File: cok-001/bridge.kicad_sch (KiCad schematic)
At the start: 48 parts, among them U7301 CXD9208GP

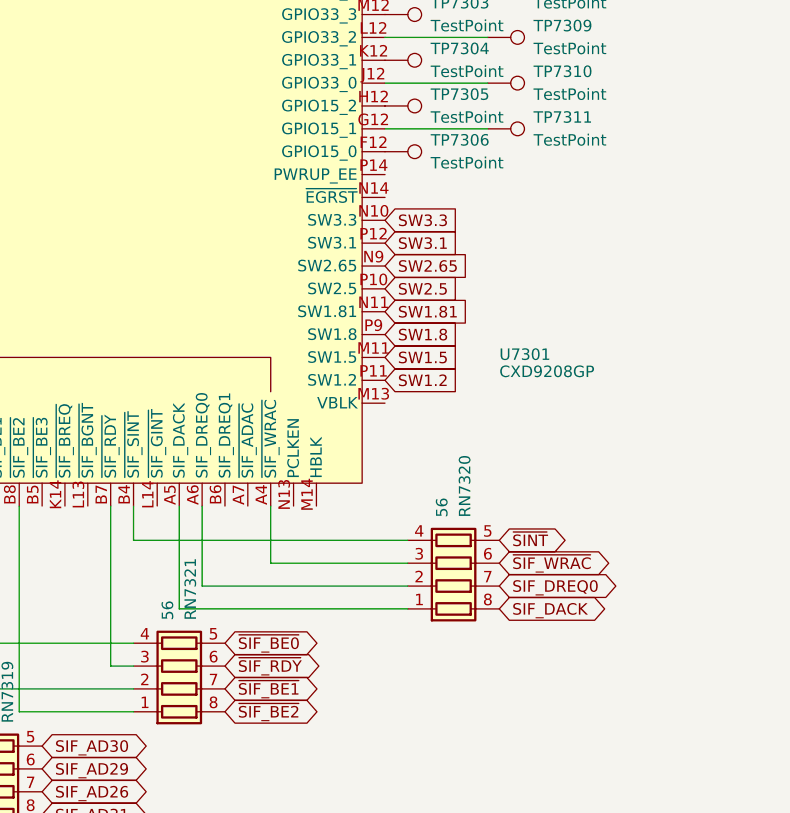
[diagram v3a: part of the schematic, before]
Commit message: ps2
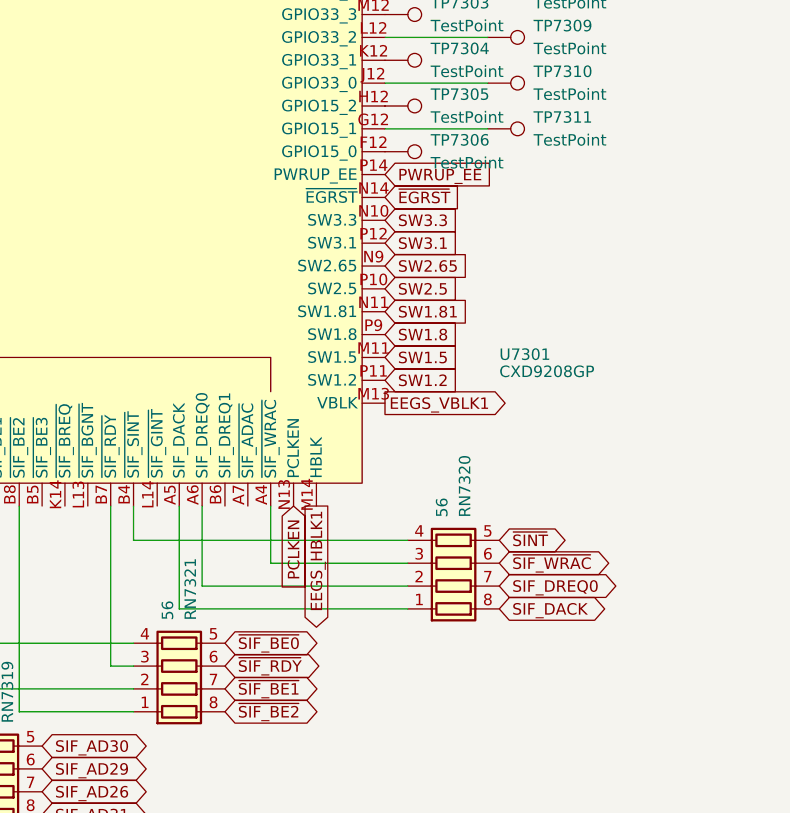
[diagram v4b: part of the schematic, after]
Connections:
- net EEGS_VBLK1: now reaches U7301.M13 (VBLK)
- net EEGS_HBLK1: now reaches U7301.M14 (HBLK)
- net PCLKEN: now reaches U7301.N13 (PCLKEN)
- net ~{EGRST}: now reaches U7301.N14 (~{EGRST})
- net PWRUP_EE: now reaches U7301.P14 (PWRUP_EE)
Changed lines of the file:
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@@
+		)
+	)
+	(global_label "EEGS_HBLK1"
+		(shape output)
+		(at 228.6 166.37 270)
+		(fields_autoplaced yes)
+		(effects
+			(font
+				(size 1.27 1.27)
+			)
+			(justify right)
+		)
+		(property "Intersheetrefs" "${INTERSHEET_REFS}"
+			(at 228.6 181.2084 90)
+			(effects
+				(font
+					(size 1.27 1.27)
+				)
+				(justify right)
+				(hide yes)
+			)
 		)
 	)
@@
 		)
 	)
+	(global_label "EEGS_VBLK1"
+		(shape output)
+		(at 236.22 154.94 0)
+		(fields_autoplaced yes)
+		(effects
+			(font
+				(size 1.27 1.27)
+			)
+			(justify left)
+		)
+		(property "Intersheetrefs" "${INTERSHEET_REFS}"
+			(at 250.8165 154.94 0)
+			(effects
+				(font
+					(size 1.27 1.27)
+				)
+				(justify left)
+				(hide yes)
+			)
+		)
+	)
 	(global_label "SIF_DACK"
 		(shape bidirectional)
@@
 		(property "Intersheetrefs" "${INTERSHEET_REFS}"
 			(at 73.66 1.3464 90)
+			(effects
+				(font
+					(size 1.27 1.27)
+				)
+				(justify left)
+				(hide yes)
+			)
+		)
+	)
+	(global_label "~{EGRST}"
+		(shape input)
+		(at 236.22 132.08 0)
+		(fields_autoplaced yes)
+		(effects
+			(font
+				(size 1.27 1.27)
+			)
+			(justify left)
+		)
+		(property "Intersheetrefs" "${INTERSHEET_REFS}"
+			(at 245.0713 132.08 0)
 			(effects
 				(font
@@
 		)
 	)
+	(global_label "PCLKEN"
+		(shape input)
+		(at 226.06 166.37 270)
+		(fields_autoplaced yes)
+		(effects
+			(font
+				(size 1.27 1.27)
+			)
+			(justify right)
+		)
+		(property "Intersheetrefs" "${INTERSHEET_REFS}"
+			(at 226.06 176.6728 90)
+			(effects
+				(font
+					(size 1.27 1.27)
+				)
+				(justify right)
+				(hide yes)
+			)
+		)
+	)
 	(global_label "SB_PCI_AD29"
 		(shape bidirectional)
@@
 			(effects
 				(font
+					(size 1.27 1.27)
+				)
+				(justify left)
+				(hide yes)
+			)
+		)
+	)
+	(global_label "PWRUP_EE"
+		(shape input)
+		(at 236.22 129.54 0)
+		(fields_autoplaced yes)
+		(effects
+			(font
+				(size 1.27 1.27)
+			)
+			(justify left)
+		)
+		(property "Intersheetrefs" "${INTERSHEET_REFS}"
+			(at 249.0627 129.54 0)
+			(effects
+				(font

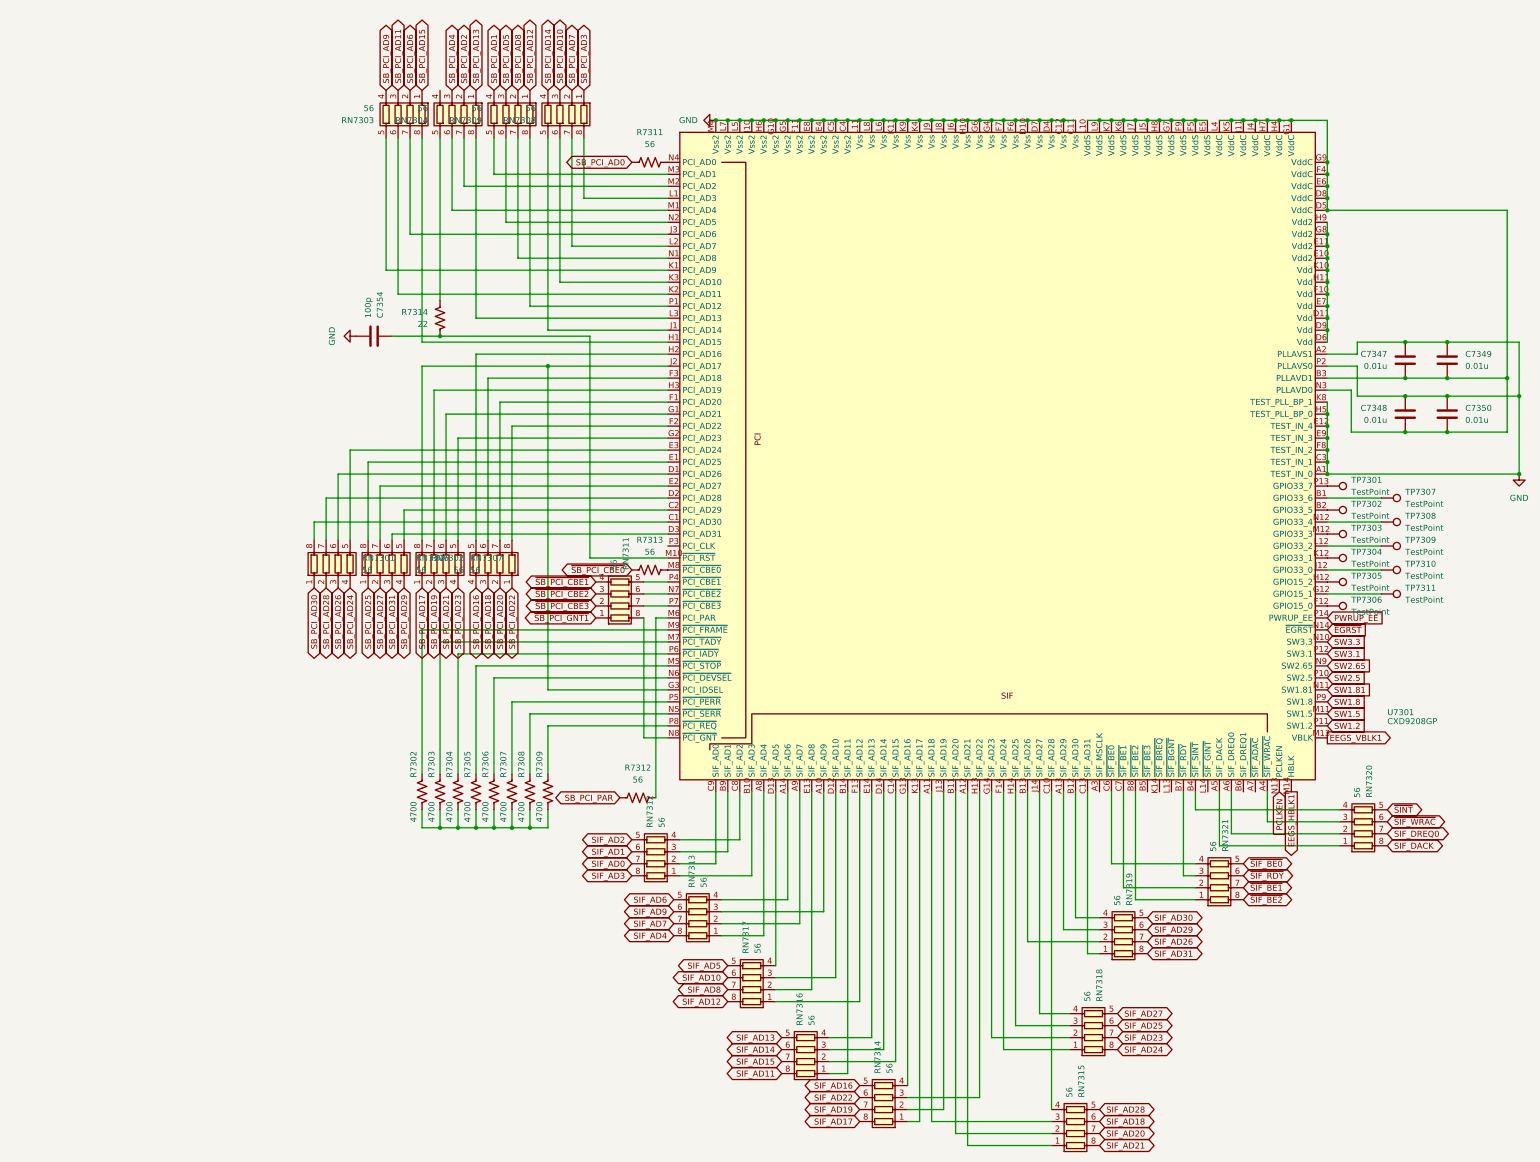
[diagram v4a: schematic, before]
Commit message: rdy
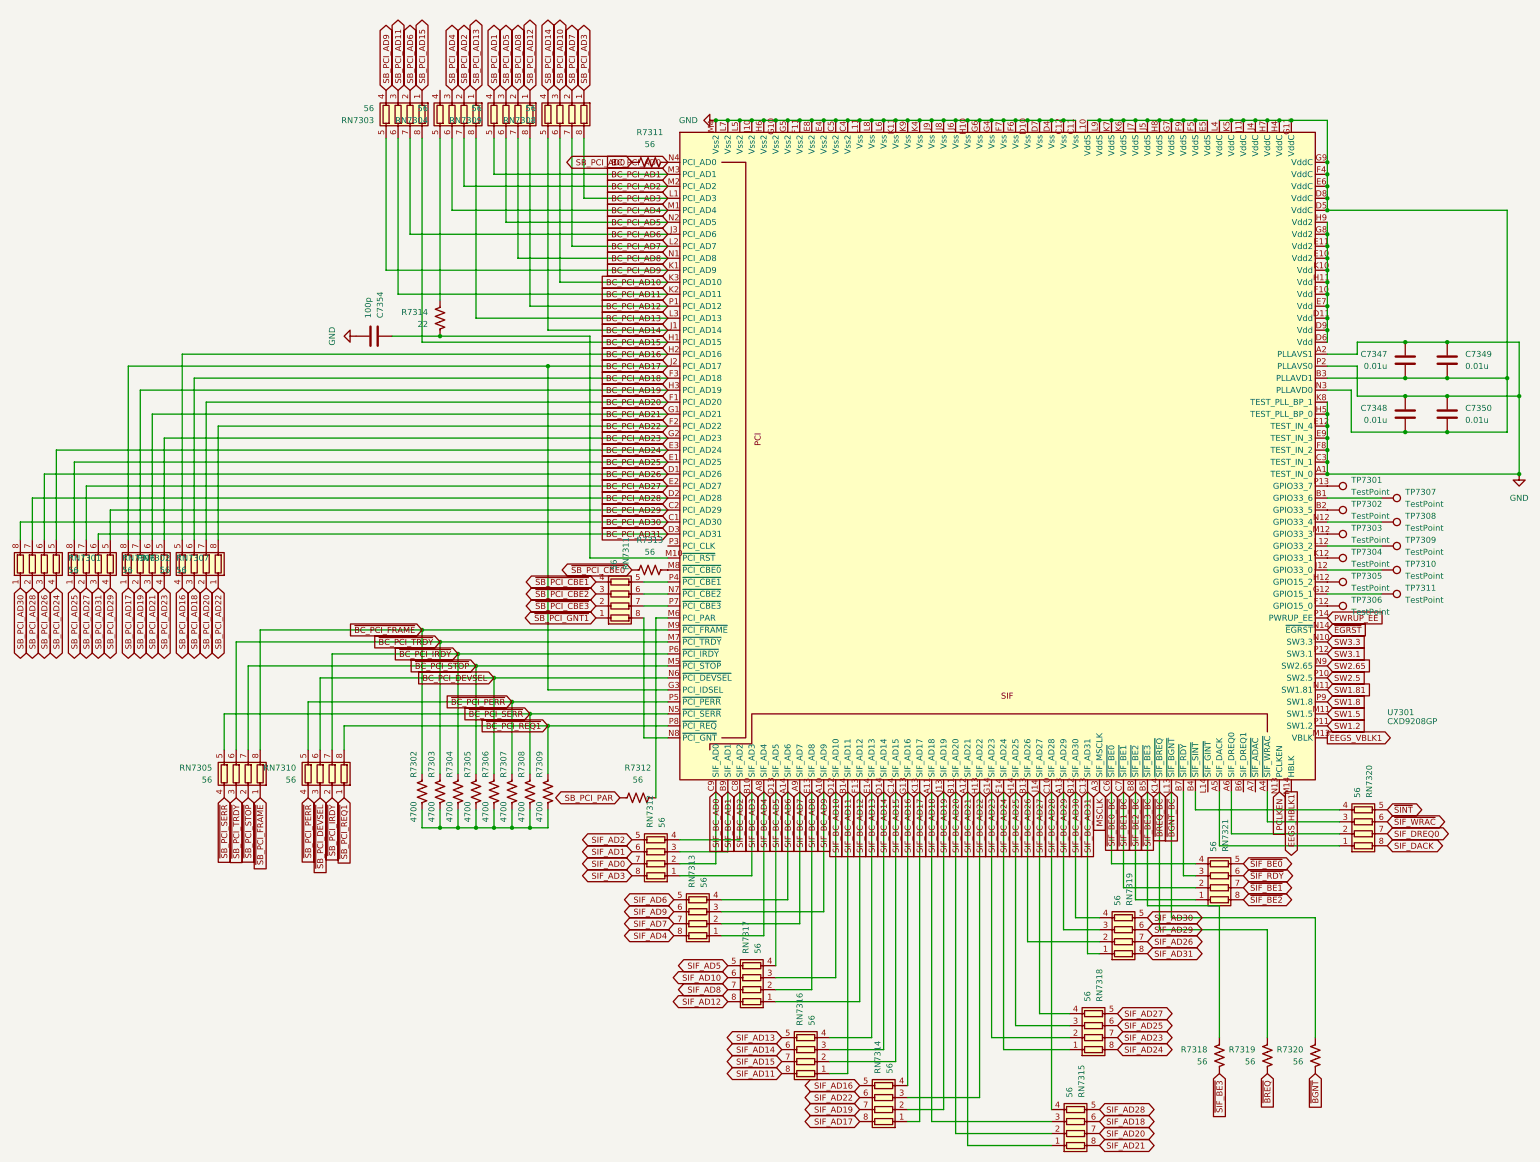
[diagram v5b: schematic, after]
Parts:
- added R7318, R7319, R7320: 56, Resistor_SMD:R_0402_1005Metric, symbol Device:R_US
- added RN7305, RN7310: 56, Resistor_SMD:R_Array_Convex_4x0402, symbol Device:R_Pack04
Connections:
- net ~{BC_PCI_STOP}: now reaches R7305.2, U7301.M5 (~{PCI_STOP})
- net ~{BC_PCI_STOP}: now also RN7305.7 (R2.2)
- net BC_PCI_AD24: now reaches RN7301.5 (R4.2), U7301.E3 (PCI_AD24)
- net BC_PCI_AD26: now reaches RN7301.6 (R3.2), U7301.D1 (PCI_AD26)
- net BC_PCI_AD28: now reaches RN7301.7 (R2.2), U7301.D2 (PCI_AD28)
- net BC_PCI_AD30: now reaches RN7301.8 (R1.2), U7301.C1 (PCI_AD30)
- net ~{BC_PCI_IRDY}: now reaches R7304.2, U7301.P6 (~{PCI_IRDY})
- net ~{BC_PCI_IRDY}: now also RN7310.7 (R2.2)
- net SIF_BC_AD4: now reaches RN7313.1 (R1.1), U7301.A8 (SIF_AD4)
- net SIF_BC_AD7: now reaches RN7313.2 (R2.1), U7301.A9 (SIF_AD7)
- net SIF_BC_AD9: now reaches RN7313.3 (R3.1), U7301.A10 (SIF_AD9)
- net SIF_BC_AD6: now reaches RN7313.4 (R4.1), U7301.A14 (SIF_AD6)
- net BC_PCI_AD1: now reaches RN7309.5 (R4.2), U7301.M3 (PCI_AD1)
- net BC_PCI_AD5: now reaches RN7309.6 (R3.2), U7301.N2 (PCI_AD5)
- net BC_PCI_AD8: now reaches RN7309.7 (R2.2), U7301.N1 (PCI_AD8)
- net BC_PCI_AD12: now reaches RN7309.8 (R1.2), U7301.P1 (PCI_AD12)
- net ~{SIF_BE2_BC}: now reaches RN7321.1 (R1.1), U7301.B8 (~{SIF_BE2})
- net ~{SIF_BE1_BC}: now reaches RN7321.2 (R2.1), U7301.C7 (~{SIF_BE1})
- net ~{SIF_BE0_BC}: now reaches RN7321.4 (R4.1), U7301.C6 (~{SIF_BE0})
- net BC_PCI_AD0: now reaches R7311.2, U7301.N4 (PCI_AD0)
- net ~{BC_PCI_SERR}: now reaches R7308.2, U7301.N5 (~{PCI_SERR})
- net ~{BC_PCI_SERR}: now also RN7305.5 (R4.2)
- net BC_PCI_DEVSEL: now reaches R7306.2, U7301.N6 (~{PCI_DEVSEL})
- net BC_PCI_DEVSEL: now also RN7310.6 (R3.2)
- net BC_PCI_AD4: now reaches RN7304.6 (R3.2), U7301.M1 (PCI_AD4)
- net BC_PCI_AD2: now reaches RN7304.7 (R2.2), U7301.M2 (PCI_AD2)
- net BC_PCI_AD13: now reaches RN7304.8 (R1.2), U7301.L3 (PCI_AD13)
- net BC_PCI_AD14: now reaches RN7308.5 (R4.2), U7301.J1 (PCI_AD14)
- net BC_PCI_AD10: now reaches RN7308.6 (R3.2), U7301.K3 (PCI_AD10)
- net BC_PCI_AD7: now reaches RN7308.7 (R2.2), U7301.L2 (PCI_AD7)
- net BC_PCI_AD3: now reaches RN7308.8 (R1.2), U7301.L1 (PCI_AD3)
- net BC_PCI_AD9: now reaches RN7303.5 (R4.2), U7301.K1 (PCI_AD9)
- net BC_PCI_AD11: now reaches RN7303.6 (R3.2), U7301.K2 (PCI_AD11)
- net BC_PCI_AD6: now reaches RN7303.7 (R2.2), U7301.J3 (PCI_AD6)
- net BC_PCI_AD15: now reaches RN7303.8 (R1.2), U7301.H1 (PCI_AD15)
- net SIF_BC_AD31: now reaches RN7319.1 (R1.1), U7301.C13 (SIF_AD31)
- net SIF_BC_AD26: now reaches RN7319.2 (R2.1), U7301.B13 (SIF_AD26)
- net SIF_BC_AD29: now reaches RN7319.3 (R3.1), U7301.A13 (SIF_AD29)
- net SIF_BC_AD30: now reaches RN7319.4 (R4.1), U7301.B12 (SIF_AD30)
- net ~{BC_PCI_TRDY}: now reaches R7303.2, U7301.M7 (~{PCI_TRDY})
- net ~{BC_PCI_TRDY}: now also RN7305.6 (R3.2)
- net BC_PCI_AD16: now reaches RN7302.5 (R4.2), U7301.H2 (PCI_AD16)
- net BC_PCI_AD18: now reaches RN7302.6 (R3.2), U7301.F3 (PCI_AD18)
- net BC_PCI_AD20: now reaches RN7302.7 (R2.2), U7301.F1 (PCI_AD20)
- net BC_PCI_AD22: now reaches RN7302.8 (R1.2), U7301.F2 (PCI_AD22)
- net ~{BC_PCI_FRAME}: now reaches R7302.2, U7301.M9 (~{PCI_FRAME})
- net ~{BC_PCI_FRAME}: now also RN7305.8 (R1.2)
- net SIF_BC_AD24: now reaches RN7318.1 (R1.1), U7301.F14 (SIF_AD24)
- net SIF_BC_AD23: now reaches RN7318.2 (R2.1), U7301.G14 (SIF_AD23)
- net SIF_BC_AD25: now reaches RN7318.3 (R3.1), U7301.H14 (SIF_AD25)
- net SIF_BC_AD27: now reaches RN7318.4 (R4.1), U7301.J14 (SIF_AD27)
- net SIF_BC_AD12: now reaches RN7317.1 (R1.1), U7301.F13 (SIF_AD12)
- net SIF_BC_AD8: now reaches RN7317.2 (R2.1), U7301.E13 (SIF_AD8)
- net SIF_BC_AD10: now reaches RN7317.3 (R3.1), U7301.D12 (SIF_AD10)
- net SIF_BC_AD5: now reaches RN7317.4 (R4.1), U7301.D13 (SIF_AD5)
- net ~{BC_PCI_REQ1}: now reaches R7309.2, U7301.P8 (~{PCI_REQ})
- net ~{BC_PCI_REQ1}: now also RN7310.8 (R1.2)
- net SIF_BC_AD3: now reaches RN7312.1 (R1.1), U7301.B10 (SIF_AD3)
- net SIF_BC_AD0: now reaches RN7312.2 (R2.1), U7301.C9 (SIF_AD0)
- net SIF_BC_AD1: now reaches RN7312.3 (R3.1), U7301.B9 (SIF_AD1)
- net SIF_BC_AD2: now reaches RN7312.4 (R4.1), U7301.C8 (SIF_AD2)
- net SIF_BC_AD11: now reaches RN7316.1 (R1.1), U7301.B14 (SIF_AD11)
- net SIF_BC_AD15: now reaches RN7316.2 (R2.1), U7301.C14 (SIF_AD15)
- net SIF_BC_AD14: now reaches RN7316.3 (R3.1), U7301.D14 (SIF_AD14)
- net SIF_BC_AD13: now reaches RN7316.4 (R4.1), U7301.E14 (SIF_AD13)
- net SIF_BC_AD17: now reaches RN7314.1 (R1.1), U7301.K13 (SIF_AD17)
- net SIF_BC_AD19: now reaches RN7314.2 (R2.1), U7301.J13 (SIF_AD19)
- net SIF_BC_AD22: now reaches RN7314.3 (R3.1), U7301.H13 (SIF_AD22)
- net SIF_BC_AD16: now reaches RN7314.4 (R4.1), U7301.G13 (SIF_AD16)
- net BC_PCI_AD23: now reaches RN7307.5 (R4.2), U7301.G2 (PCI_AD23)
- net BC_PCI_AD21: now reaches RN7307.6 (R3.2), U7301.G1 (PCI_AD21)
- net BC_PCI_AD19: now reaches RN7307.7 (R2.2), U7301.H3 (PCI_AD19)
- net BC_PCI_AD17: now reaches RN7307.8 (R1.2), U7301.G3 (PCI_IDSEL), U7301.J2 (PCI_AD17)
- net ~{BC_PCI_PERR}: now reaches R7307.2, U7301.P5 (~{PCI_PERR})
- net ~{BC_PCI_PERR}: now also RN7310.5 (R4.2)
- net SIF_BC_AD21: now reaches RN7315.1 (R1.1), U7301.A12 (SIF_AD21)
- net SIF_BC_AD20: now reaches RN7315.2 (R2.1), U7301.B11 (SIF_AD20)
- net SIF_BC_AD18: now reaches RN7315.3 (R3.1), U7301.A11 (SIF_AD18)
- net SIF_BC_AD28: now reaches RN7315.4 (R4.1), U7301.C10 (SIF_AD28)
- net BC_PCI_AD29: now reaches RN7306.5 (R4.2), U7301.C2 (PCI_AD29)
- net BC_PCI_AD31: now reaches RN7306.6 (R3.2), U7301.D3 (PCI_AD31)
- net BC_PCI_AD27: now reaches RN7306.7 (R2.2), U7301.E2 (PCI_AD27)
- net BC_PCI_AD25: now reaches RN7306.8 (R1.2), U7301.E1 (PCI_AD25)
- net MSCLK: now reaches U7301.A3 (SIF_MSCLK)
- net ~{SIF_BE3_BC}: now reaches U7301.B5 (~{SIF_BE3})
- net ~{SIF_BE3_BC}: now also R7318.2
- net ~{BREQ_BC}: now reaches U7301.K14 (~{SIF_BREQ})
- net ~{BREQ_BC}: now also R7319.2
- net ~{BGNT_BC}: now reaches U7301.L13 (~{SIF_BGNT})
- net ~{BGNT_BC}: now also R7320.2
- new net ~{BGNT}: R7320.1
- new net ~{BREQ}: R7319.1
- new net ~{SB_PCI_DEVSEL}: RN7310.3 (R3.1)
- new net ~{SB_PCI_FRAME}: RN7305.1 (R1.1)
- new net ~{SB_PCI_IRDY}: RN7310.2 (R2.1)
- new net ~{SB_PCI_PERR}: RN7310.4 (R4.1)
- new net ~{SB_PCI_REQ1}: RN7310.1 (R1.1)
- new net ~{SB_PCI_SERR}: RN7305.4 (R4.1)
- new net ~{SB_PCI_STOP}: RN7305.2 (R2.1)
- new net ~{SB_PCI_TRDY}: RN7305.3 (R3.1)
- new net ~{SIF_BE3}: R7318.1
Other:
- moved on the sheet: RN7301, RN7302, RN7306, RN7307
